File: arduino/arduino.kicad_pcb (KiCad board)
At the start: 2 copper layers, 14 parts, among them IC1 ATMEGA328P-P, P1 CONN_6, P2 CONN_2, P3 CONN_6, P4 CONN_6, P5 CONN_1, P6 CONN_6, Q1 16MHz, U1 RFM12B

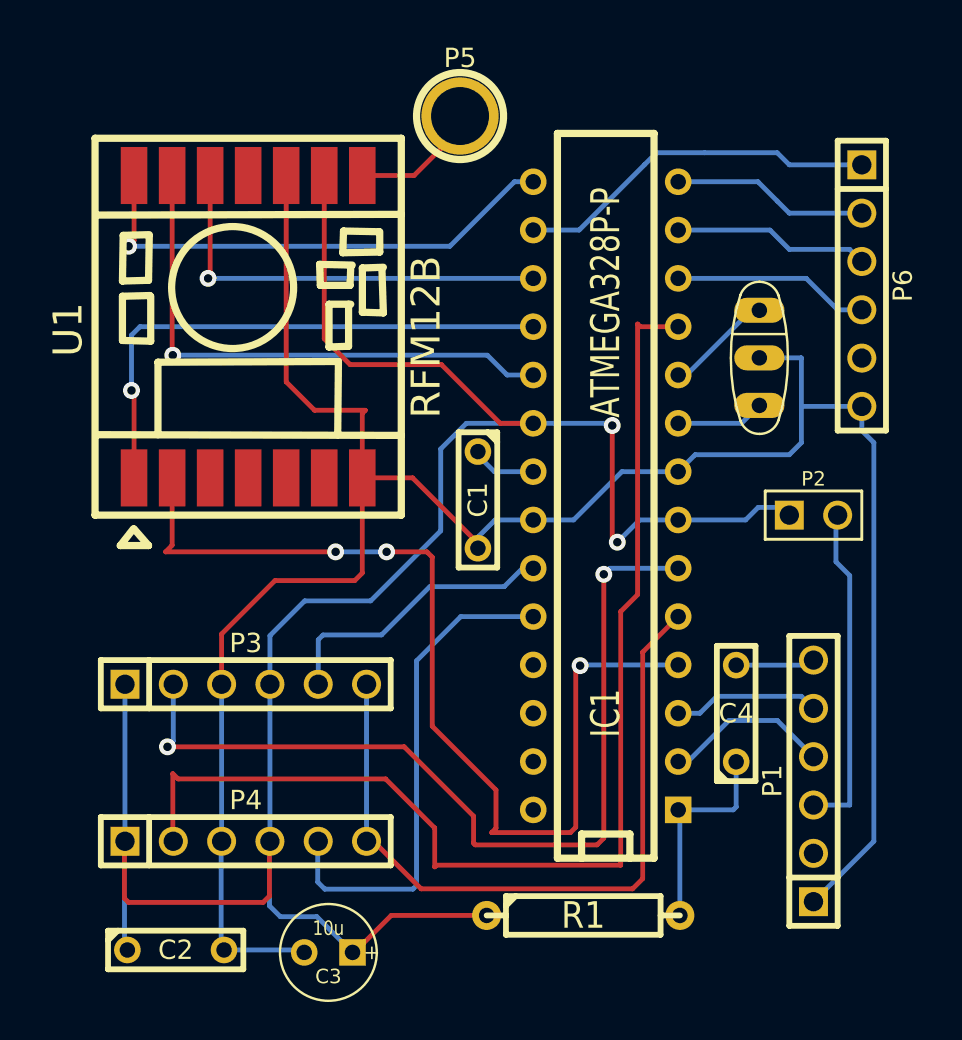
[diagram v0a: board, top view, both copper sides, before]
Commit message: more pcb work
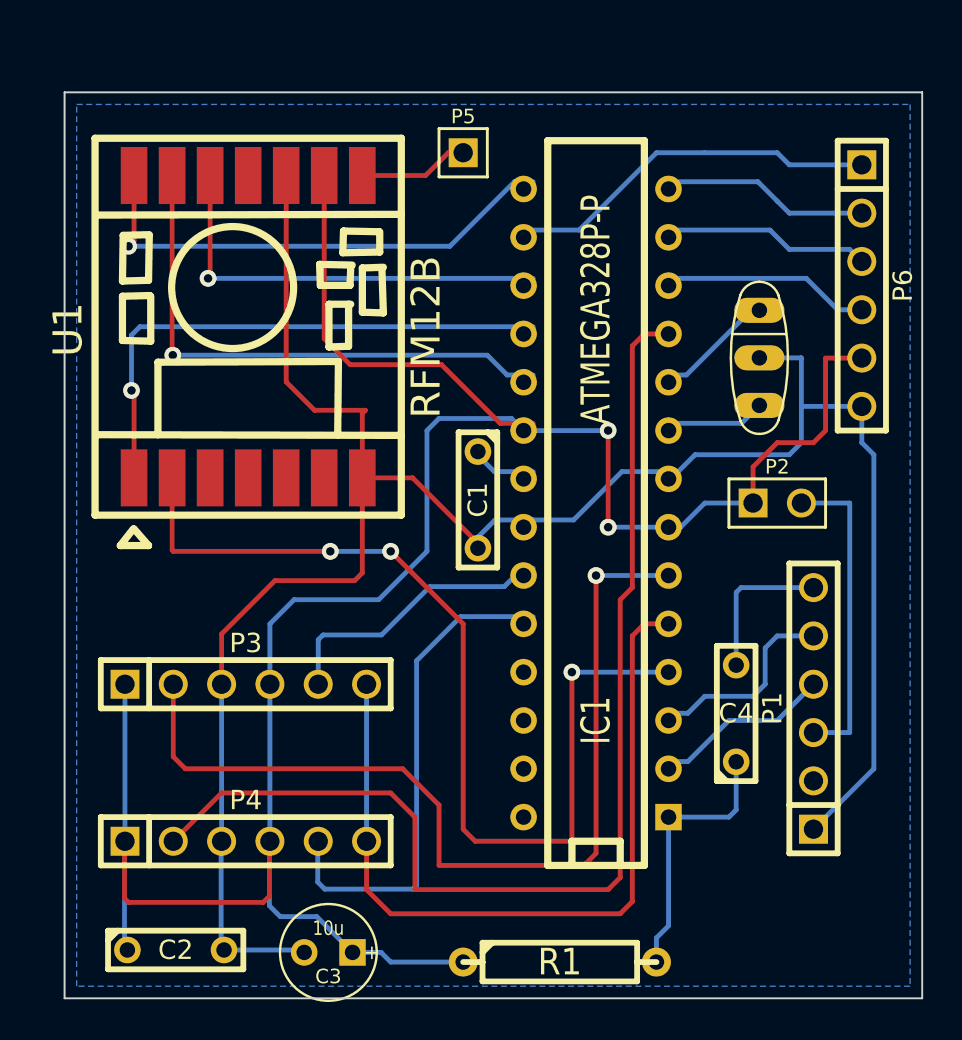
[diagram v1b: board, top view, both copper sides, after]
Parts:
- P5: footprint 1pin -> PIN_ARRAY_1
- moved P1 3.81 mm to (111.1, 143.5)
- moved R1 2.74 mm to (97.8, 156.8)
- moved P2 2.01 mm to (109.2, 132.7)
- moved P5 1.94 mm to (92.7, 114.3)
- moved IC1 0.64 mm to (99.7, 132.7)
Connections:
- P6 pad 5: (no net) -> VCC
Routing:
- net VCC: track 118.8 -> 128.1 mm
- net N-000008: track 4.17 -> 7.99 mm
- net GND: track 118.8 -> 115.0 mm
- net N-0000021: track 11.1 -> 14.1 mm
- net N-0000012: track 38.4 -> 41.2 mm
- net N-000009: track 7.74 -> 9.91 mm
- net N-000007: track 47.4 -> 48.9 mm, vias 2 -> 1
- net N-000006: track 17.9 -> 16.5 mm
- net N-0000010: track 60.9 -> 59.5 mm
- net N-0000035: track 6.85 -> 5.80 mm
- net N-0000027: track 52.4 -> 51.4 mm
- added copper zone on B.Cu, net (none)
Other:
- board outline added: 45.1 x 47.6 mm
